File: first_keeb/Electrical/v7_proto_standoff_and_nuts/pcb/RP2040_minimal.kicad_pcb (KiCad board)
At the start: 2 copper layers, 77.7 x 77.5 mm, 71 parts, among them P1 USB-TYPE-C-016, Q1 SN74LV1T34DBV, SW1 SKRKAGE020, SW2 PTS647 SN70 SMTR2 LFS, SW3 PTS647 SN70 SMTR2 LFS, U1 NCP1117-3.3_SOT223, U2 LM4040DBZ-3, U3 PRTR5V0U2X, U4 W25Q32JVSS, U5 RP2040, Y1 ABM7-12.000MHZ-D2Y-T

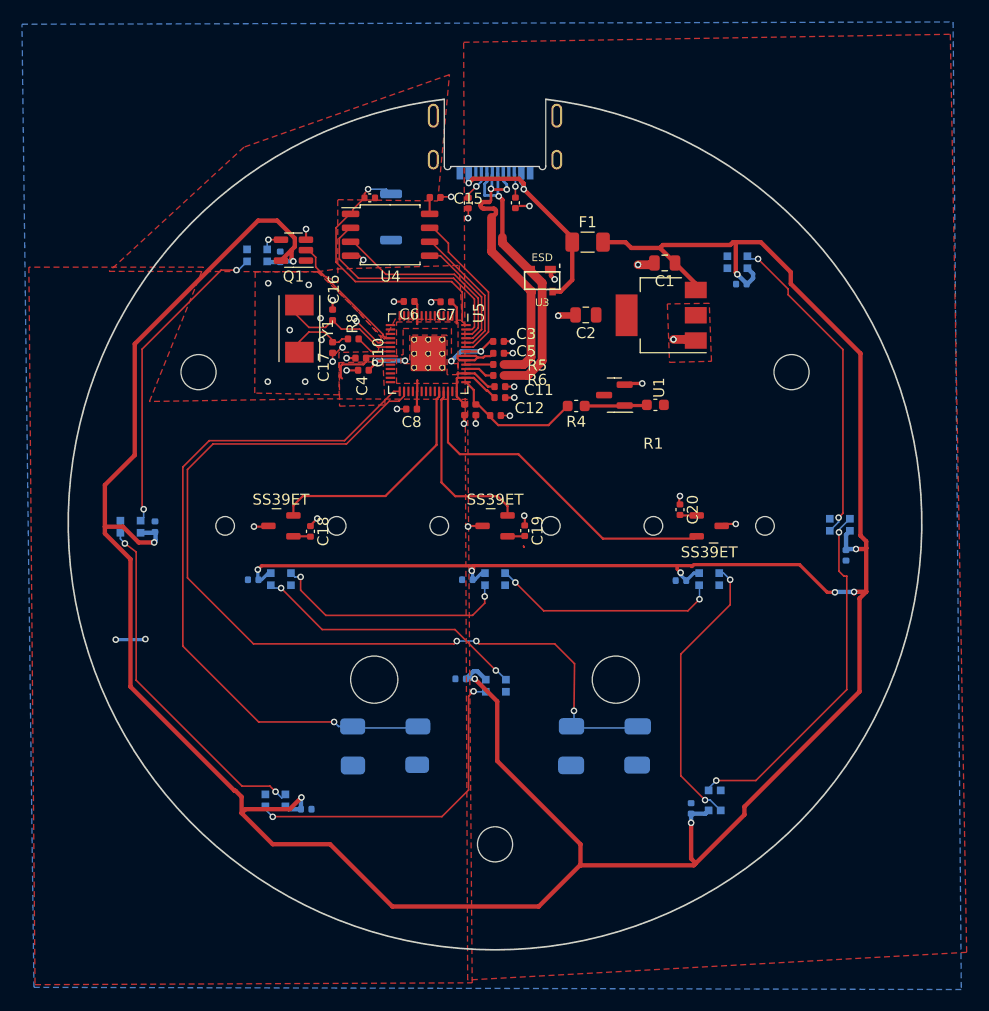
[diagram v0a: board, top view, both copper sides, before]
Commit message: case with mid mount
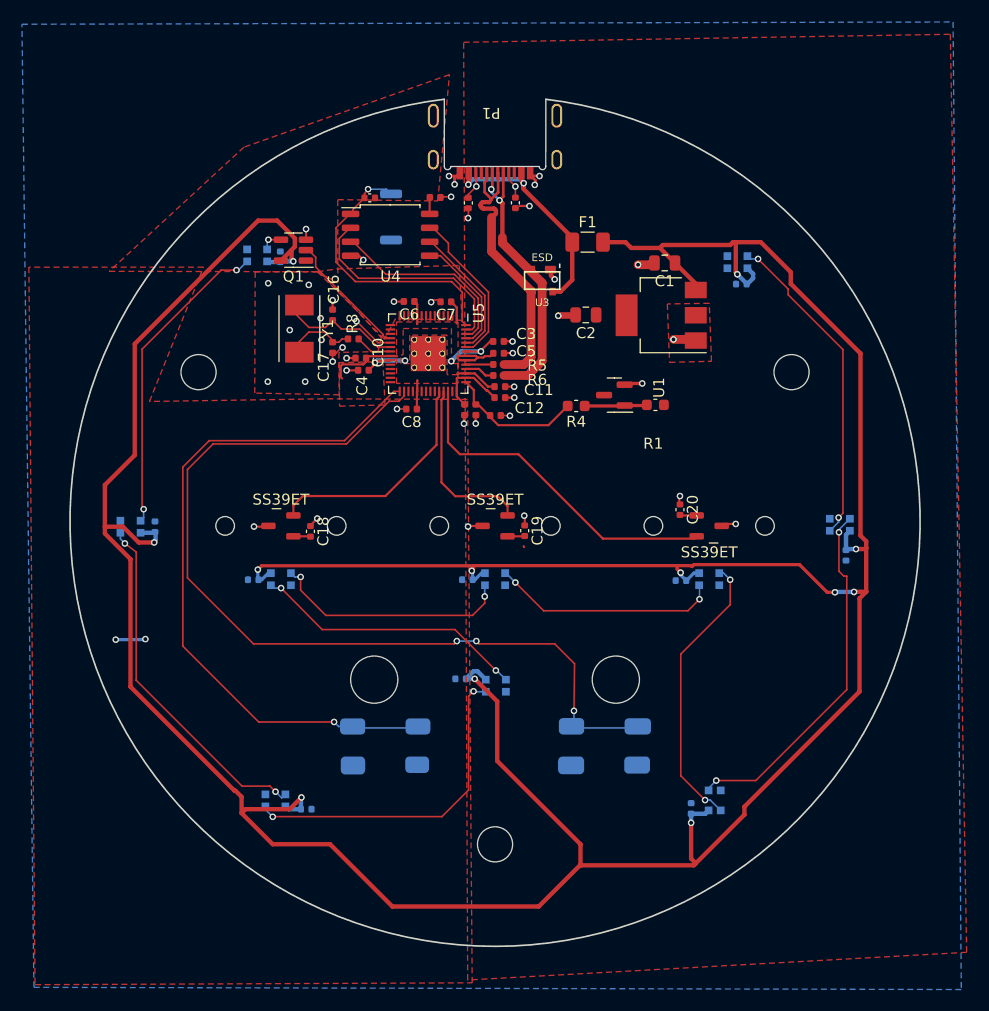
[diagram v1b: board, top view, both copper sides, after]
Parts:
- P1: moved to F.Cu
- turned P1 to 180 degrees
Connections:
- R2 pad 1: Net-(P1-CC2) -> Net-(P1-CC1)
- R3 pad 1: Net-(P1-CC1) -> Net-(P1-CC2)
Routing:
- net GND: track 33.1 -> 37.3 mm, vias 39 -> 43
- net /USB_D-: track 26.3 -> 25.6 mm, vias 1 -> 2
- net /USB_D+: track 25.7 -> 26.0 mm, vias 2 -> 0
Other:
- board size 77.7 x 77.5 mm -> 77.4 x 77.1 mm
